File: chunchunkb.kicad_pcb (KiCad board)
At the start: 2 copper layers, 143.7 x 121.4 mm, 124 parts, among them J1 BATT, J2 OLED, SW1 SW_Push, SW10 SW_Push, SW11 SW_Push, SW12 SW_Push, SW13 SW_Push, SW14 SW_Push, SW15 SW_Push, SW16 SW_Push, SW17 SW_Push, SW18 SW_Push, SW19 SW_Push, SW2 SW_Push, SW20 SW_Push, SW21 SW_Push, SW22 SW_Push, SW23 SW_Push, SW24 SW_Push, SW25 SW_Push, SW26 SW_Push, SW27 SW_Push, SW28 SW_Push, SW29 SW_Push, SW3 SW_Push, SW30 SW_Push, SW31 EC11, SW32 SW_Push, SW33 SW_Push, SW34 SW_Push, SW35 SW_Push, SW36 SW_Push, SW4 SW_Push, SW5 SW_Push, SW6 SW_Push, SW7 SW_Push, SW8 SW_Push, SW9 SW_Push

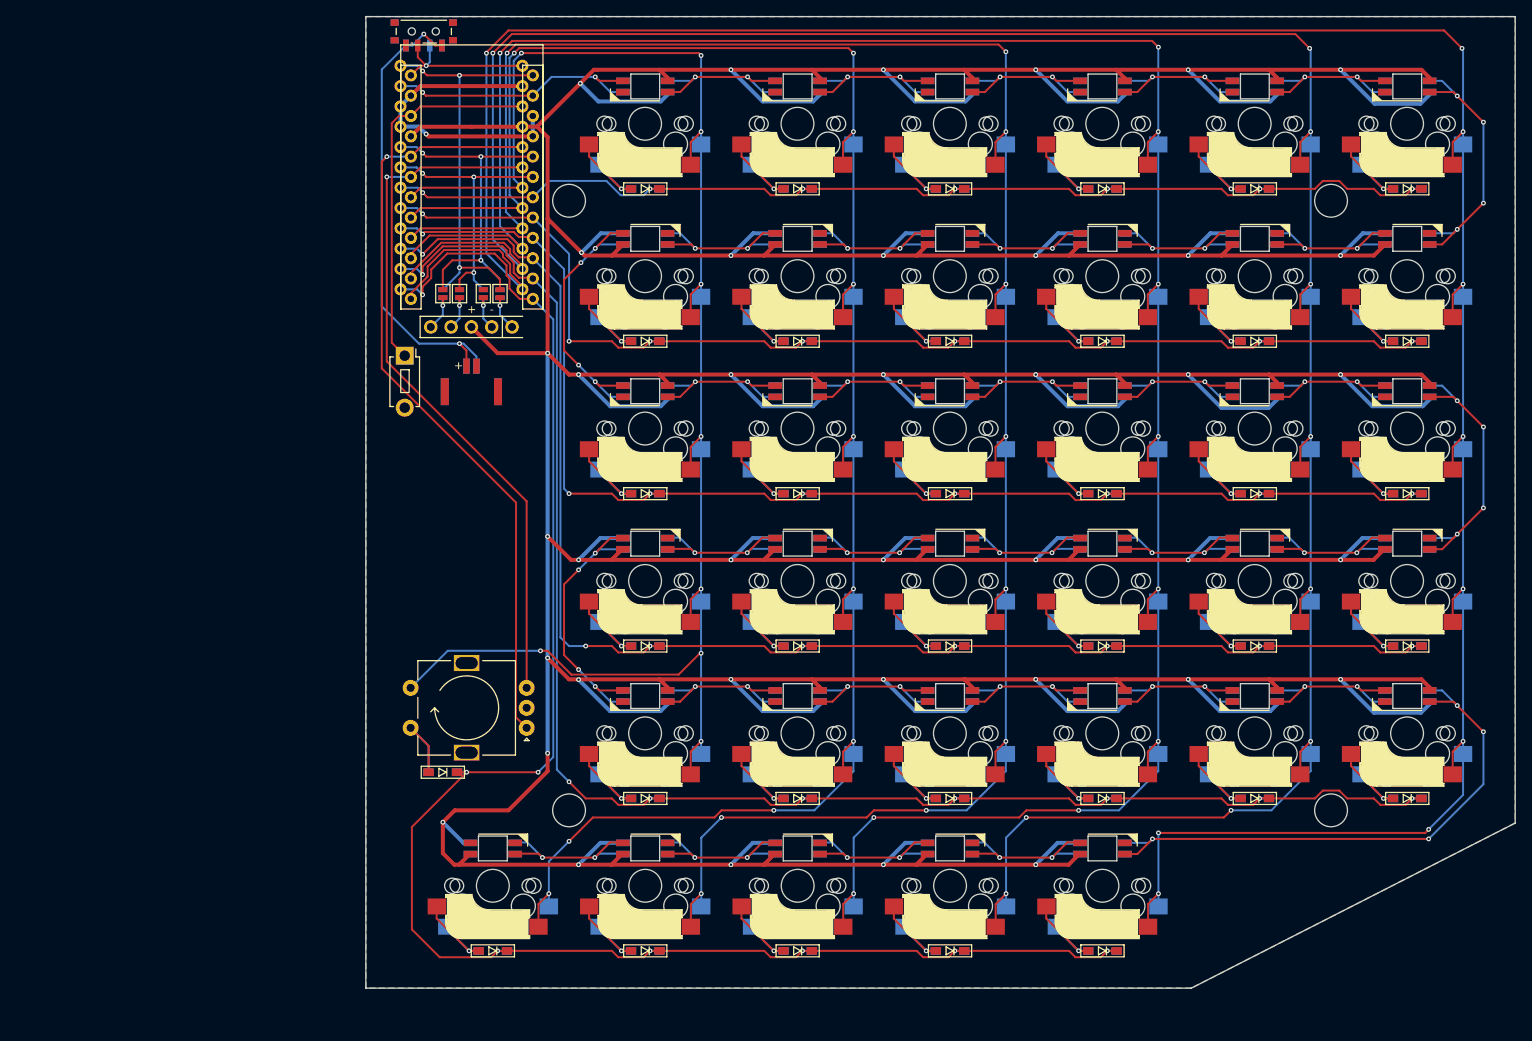
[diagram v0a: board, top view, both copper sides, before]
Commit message: Merge pull request #2 from qwerty22121998/feat/rev2
feat: rev 2 board
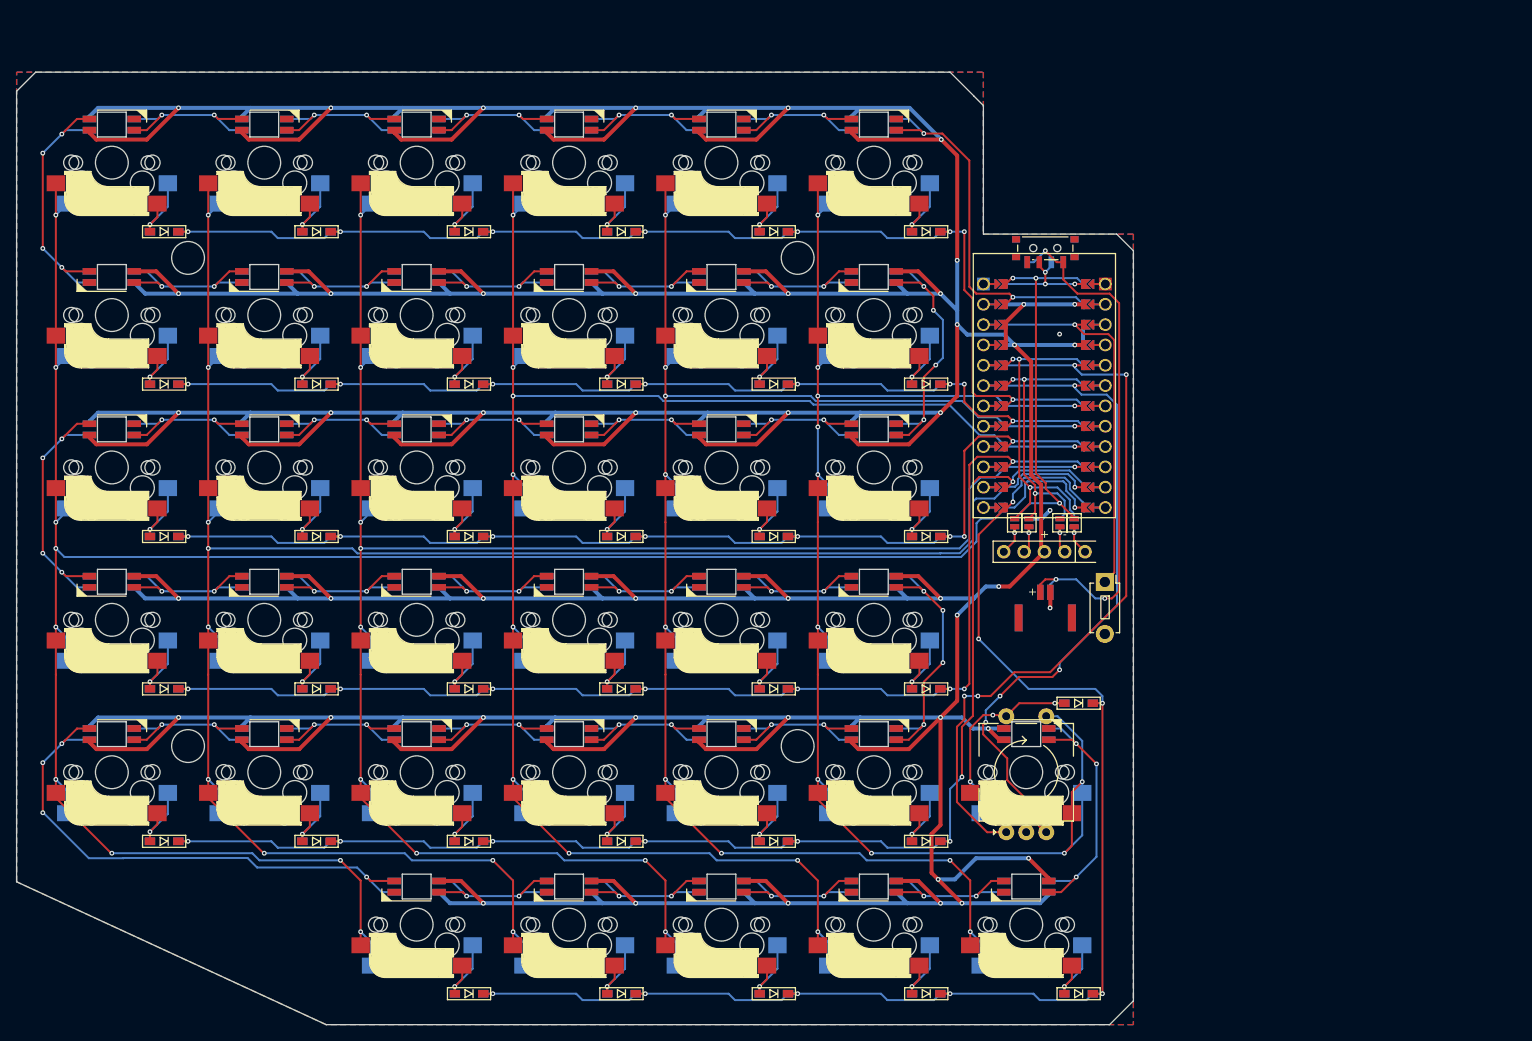
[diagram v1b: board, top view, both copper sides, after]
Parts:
- added LED36: YS-SK6812MINI-E, chunchunkb:YS-SK6812MINI-E, F.Cu at (161.9, 109.5)
- SW31: footprint chunchunkb:EC11_Switch -> chunchunkb:EC11_MX_Hybrid
- U1: footprint chunchunkb:ProMicro DUAL -> chunchunkb:ProMicro_DUAL
- moved LED7 162.0 mm to (47.6, 52.4), turned to 0 degrees
- moved LED19 162.0 mm to (47.6, 90.5), turned to 0 degrees
- moved LED18 162.0 mm to (47.6, 71.4), turned to 180 degrees
- moved LED30 162.0 mm to (47.6, 109.5), turned to 180 degrees
- moved LED6 162.0 mm to (47.6, 33.3), turned to 180 degrees
- moved SW12 162.0 mm to (47.6, 57.1)
- moved SW18 162.0 mm to (47.6, 76.2)
- moved SW24 162.0 mm to (47.6, 95.2)
- moved SW30 162.0 mm to (47.6, 114.3)
- moved SW6 162.0 mm to (47.6, 38.1)
- moved D12 155.5 mm to (54.2, 65.8)
- moved D18 155.5 mm to (54.2, 84.8)
- moved D24 155.5 mm to (54.2, 103.9)
- moved D30 155.5 mm to (54.2, 122.9)
- moved D6 155.5 mm to (54.2, 46.7)
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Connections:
- LED35 pad 2: unconnected-(LED35-DOUT-Pad2) -> Net-(LED35-DOUT)
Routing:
- net COL 5: track 346.9 -> 285.3 mm
- net COL 4: track 319.0 -> 265.8 mm
- net COL 3: track 293.6 -> 246.0 mm
- net COL 2: track 268.5 -> 224.2 mm
- net ROW 5: track 217.3 -> 176.5 mm
- net COL 1: track 243.8 -> 204.1 mm
- net ROW 4: track 205.7 -> 170.5 mm
- net Net-(LED35-DOUT): track 0.00 -> 34.5 mm, vias 0 -> 3
- net ROW 3: track 187.1 -> 153.4 mm
- net ROW 2: track 168.7 -> 136.8 mm
- net ROW 1: track 152.0 -> 128.3 mm
- net GND: track 38.5 -> 23.3 mm, vias 1 -> 5
- net SW31B: track 13.0 -> 26.9 mm, vias 0 -> 3
- net LED: track 33.7 -> 47.1 mm
- net COL 0: track 205.9 -> 193.1 mm, vias 9 -> 11
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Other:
- board size 143.7 x 121.4 mm -> 139.6 x 119.1 mm
